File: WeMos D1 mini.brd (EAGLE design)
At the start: 25.4 x 28.9 mm, 19 parts

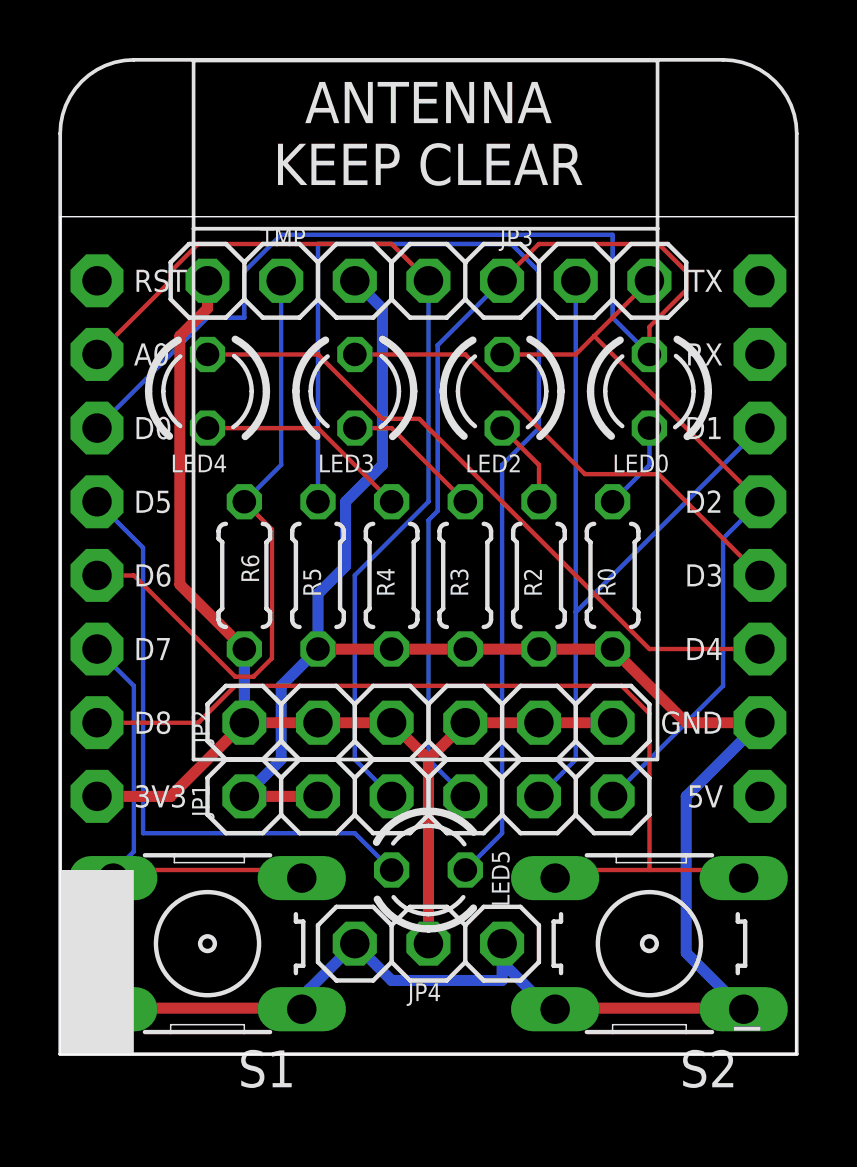
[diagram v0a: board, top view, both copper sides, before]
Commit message: 1st prototype candidate 1
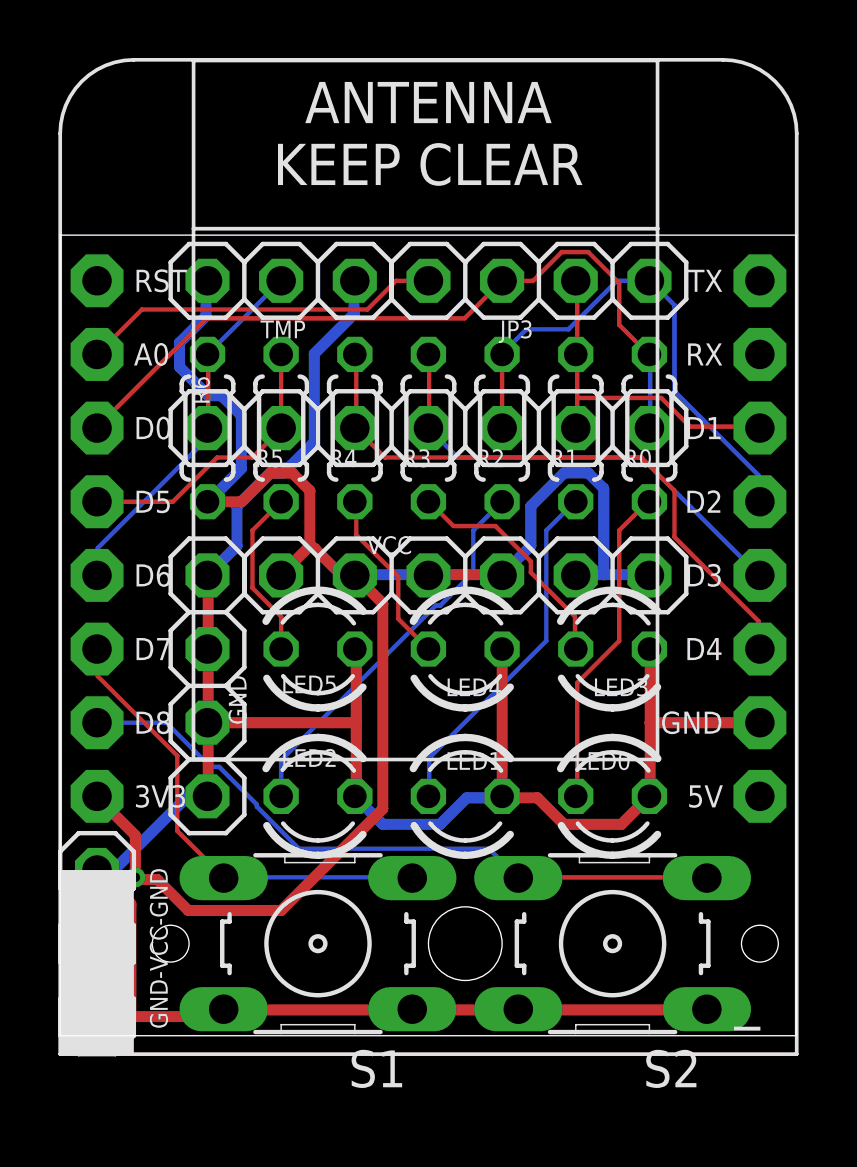
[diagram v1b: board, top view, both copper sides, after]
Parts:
- removed JP2: (no value), pinhead_v2:1X06/OCT
- removed JP4: (no value), pinhead_v2:1X03/OCT
- added GND: (no value), pinhead_v2:1X04/OCT
- added GND-VCC-GND: (no value), pinhead_v2:1X03/OCT
- added LED1: (no value), led:LED3MM
- added R1: (no value), resistor:0204/5
- added VCC: (no value), pinhead_v2:1X06/OCT
- JP1: device pinhead_v2:1X06/OCT -> pinhead_v2:1X07/OCT
- R6: value (none) -> 10K
- moved LED2 15.3 mm to (8.89, 8.89), turned to 0 degrees
- moved LED0 14.0 mm to (19.1, 8.89), turned to 0 degrees
- moved JP1 12.7 mm to (12.7, 21.6), turned to 180 degrees
- moved LED3 12.6 mm to (19.1, 14.0), turned to 0 degrees
- moved LED4 12.6 mm to (14.0, 14.0), turned to 0 degrees
- moved LED5 8.52 mm to (8.89, 14.0)
- moved R0 5.24 mm to (20.3, 21.6)
- moved R2 5.24 mm to (15.2, 21.6)
- moved R3 5.24 mm to (12.7, 21.6)
- moved R4 5.24 mm to (10.2, 21.6)
- moved R5 5.24 mm to (7.62, 21.6)
- moved R6 5.24 mm to (5.08, 21.6)
- moved S1 3.81 mm to (8.89, 3.81)
- moved S2 1.27 mm to (19.1, 3.81)
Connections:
- new net N$6: LED0.A, R0.1
- net A0: no longer JP1.3
- net D0: now also JP1.1, R0.2; no longer JP1.4, LED0.A
- net D1: now also JP1.2, R1.2; no longer JP1.5
- net D2: now also JP1.3, R2.2; no longer JP1.6, LED2.A
- net D3: now also JP1.4, R3.2; no longer LED3.A
- net D4: now also JP1.5, R4.2; no longer LED4.A
- net D5: now also JP1.6, R5.2; no longer LED5.A
- net D6: now also JP1.7
- net GND: now also GND-VCC-GND.1, GND-VCC-GND.3, GND.1, GND.2, GND.3, GND.4, LED0.K, LED1.K, LED2.K, LED3.K, LED4.K, LED5.K; no longer JP1.1, JP1.2, JP4.1, JP4.3, R0.1, R2.1, R3.1, R4.1, R5.1
- net N$1: now also LED5.A, R5.1; no longer LED0.K, R0.2
- net N$2: now also LED4.A, R4.1; no longer LED2.K, R2.2
- net N$3: now also LED3.A, R3.1; no longer LED3.K, R3.2
- net N$4: now also LED2.A, R2.1; no longer LED4.K, R4.2
- net N$5: now also LED1.A, R1.1; no longer LED5.K, R5.2
- net VCC: now also GND-VCC-GND.2, VCC.1, VCC.2, VCC.3, VCC.4, VCC.5, VCC.6; no longer JP2.1, JP2.2, JP2.3, JP2.4, JP2.5, JP2.6, JP4.2
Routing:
- net D0: track 56.1 -> 26.4 mm
- net N$5: track 38.6 -> 12.3 mm
- net A0: track 33.1 -> 12.5 mm
- net VCC: track 42.8 -> 60.9 mm, vias 0 -> 1
- net D1: track 27.3 -> 11.9 mm
- net GND: track 76.3 -> 87.8 mm
- net N$6: track 0.00 -> 11.3 mm
- net D5: track 21.2 -> 9.96 mm
- net D8: track 32.3 -> 23.3 mm
- net D6: track 21.7 -> 12.8 mm
- net D2: track 26.5 -> 17.9 mm
- net N$4: track 7.40 -> 13.4 mm
- net N$3: track 4.86 -> 8.04 mm
- net N$2: track 3.07 -> 6.16 mm
- net N$1: track 3.07 -> 5.90 mm
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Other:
- board size 25.4 x 28.9 mm -> 25.4 x 27.6 mm
